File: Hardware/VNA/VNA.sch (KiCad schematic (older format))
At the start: 26 parts, among them J1 USB_B_Micro, J2 USB_A, J3 Conn_ARM_SWD, J4 SMA, J5 SMA, J6 UART, U1 TPD2S017, U2 TPD2S017

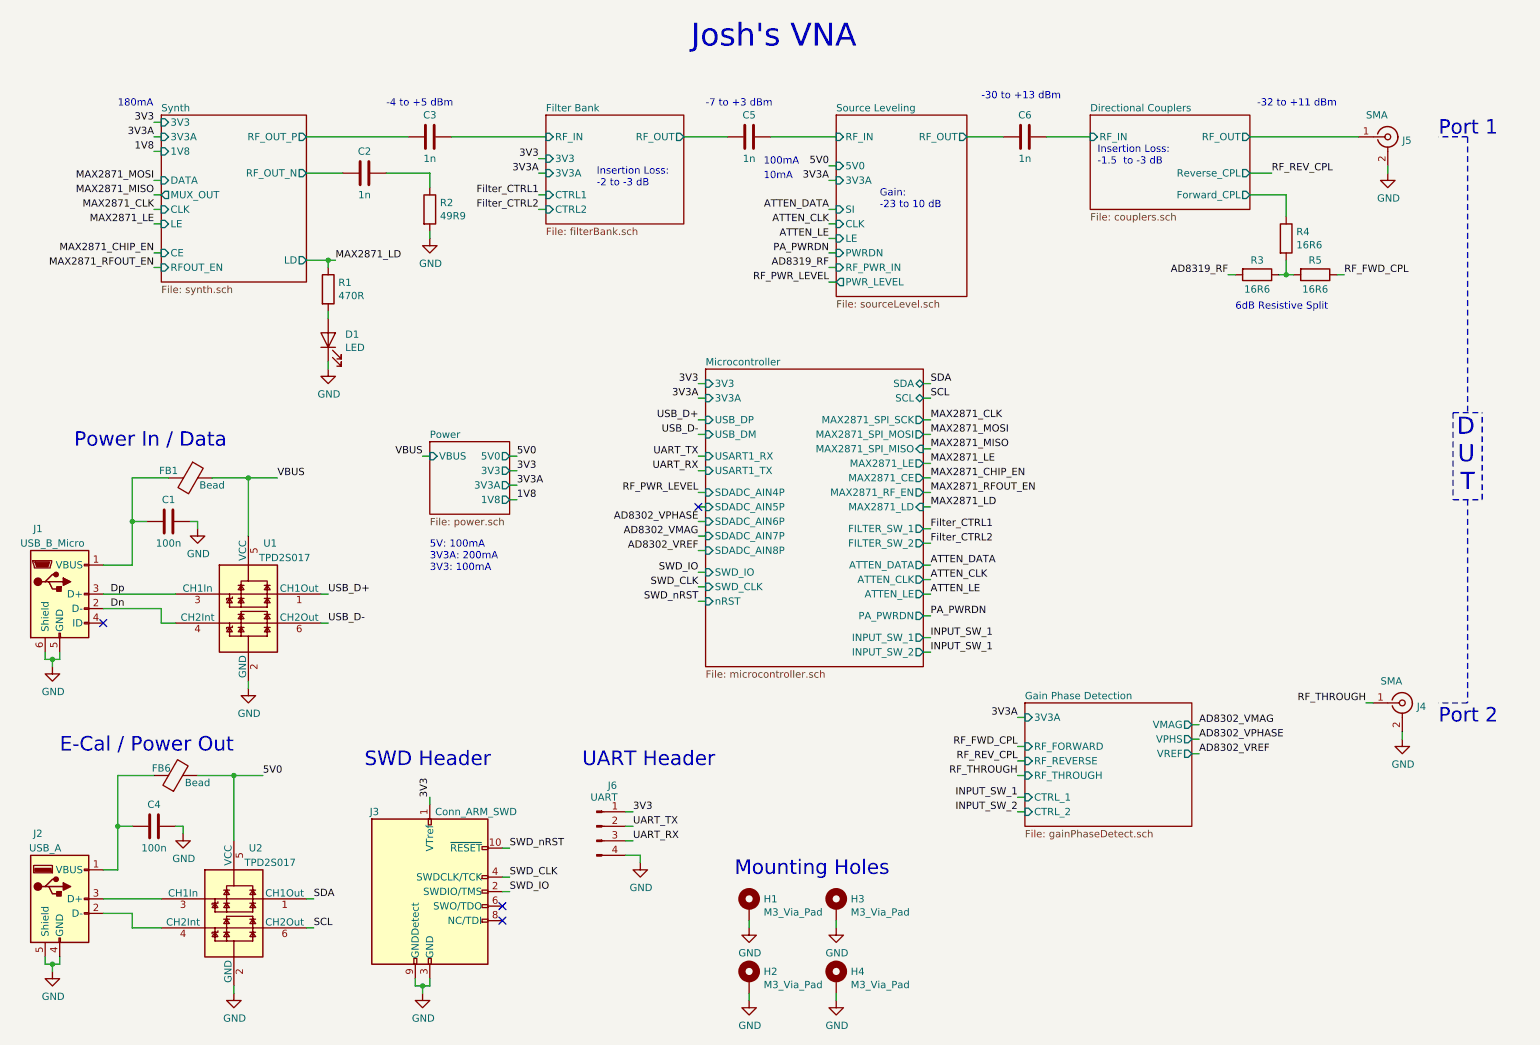
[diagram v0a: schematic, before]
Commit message: More schematic changes + updated functionals
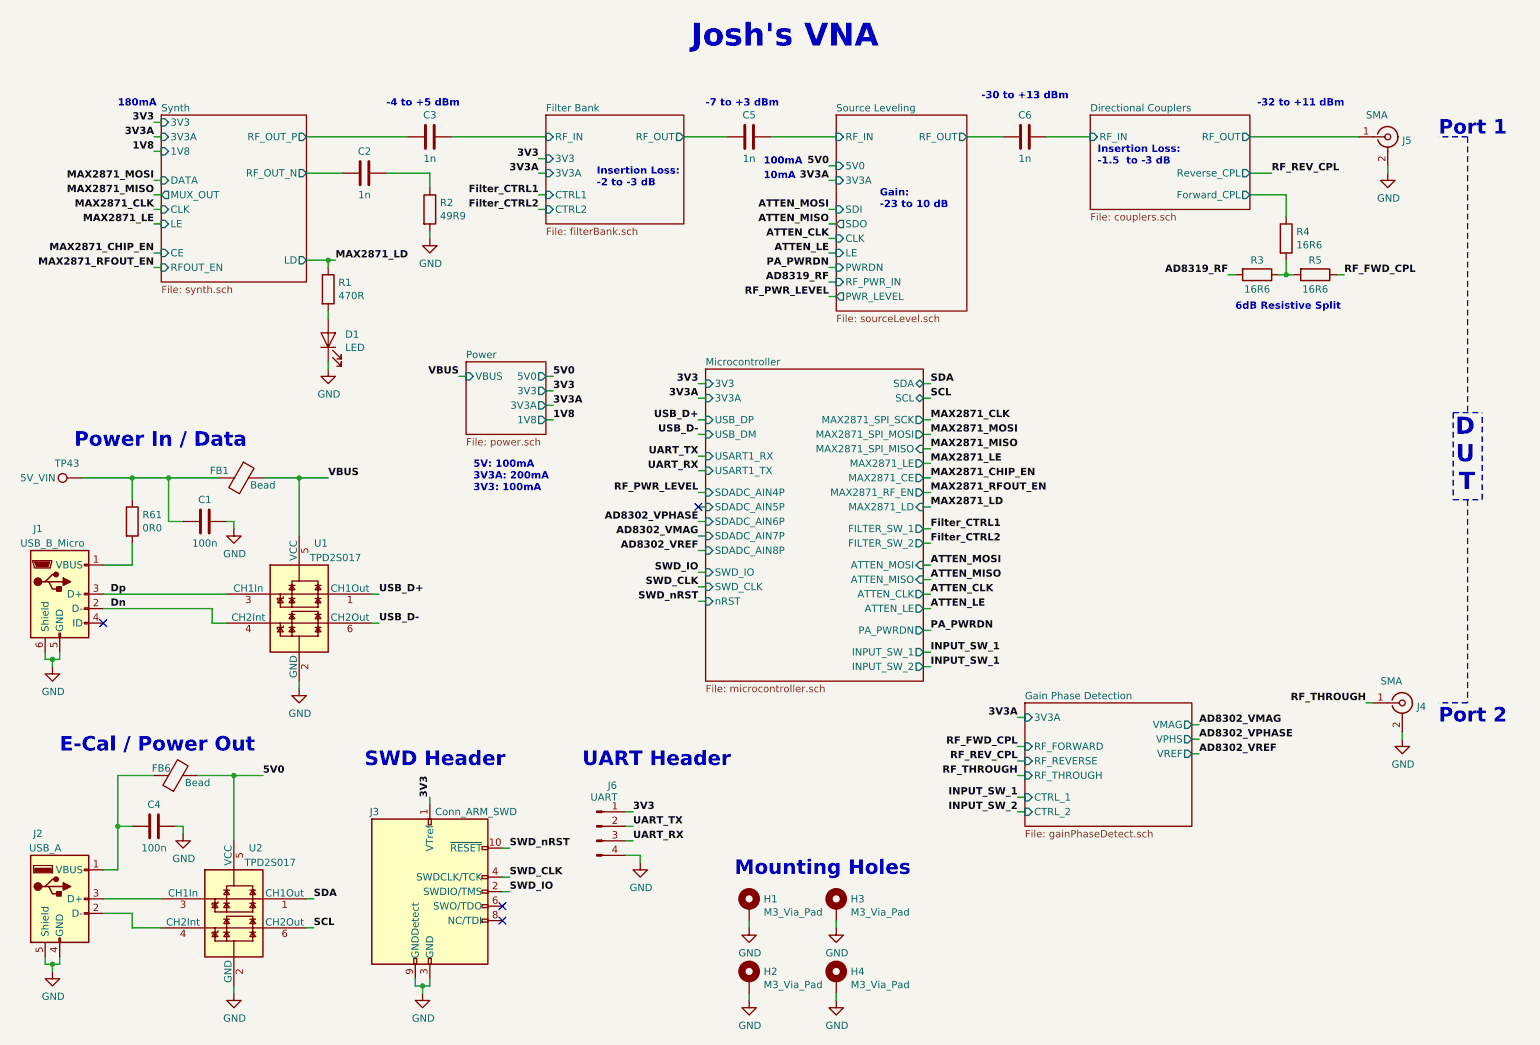
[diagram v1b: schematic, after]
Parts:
- added R61: 0R0, Resistor_SMD:R_0603_1608Metric, symbol Device:R
- added TP43: 5V_VIN, VNA_Footprints:TestPoint_Loop_D1.80mm_Drill1.0mm_Beaded_RED, symbol Connector:TestPoint
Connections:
- net at C1.1, FB1.2: now also R61.1, TP43.1; no longer J1.1 (VBUS)
- new net: J1.1 (VBUS), R61.2
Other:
- moved on the sheet: C1, FB1, U1
